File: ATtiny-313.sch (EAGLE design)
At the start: 16 parts, among them IC1 REG1117, IC2 ATtiny85

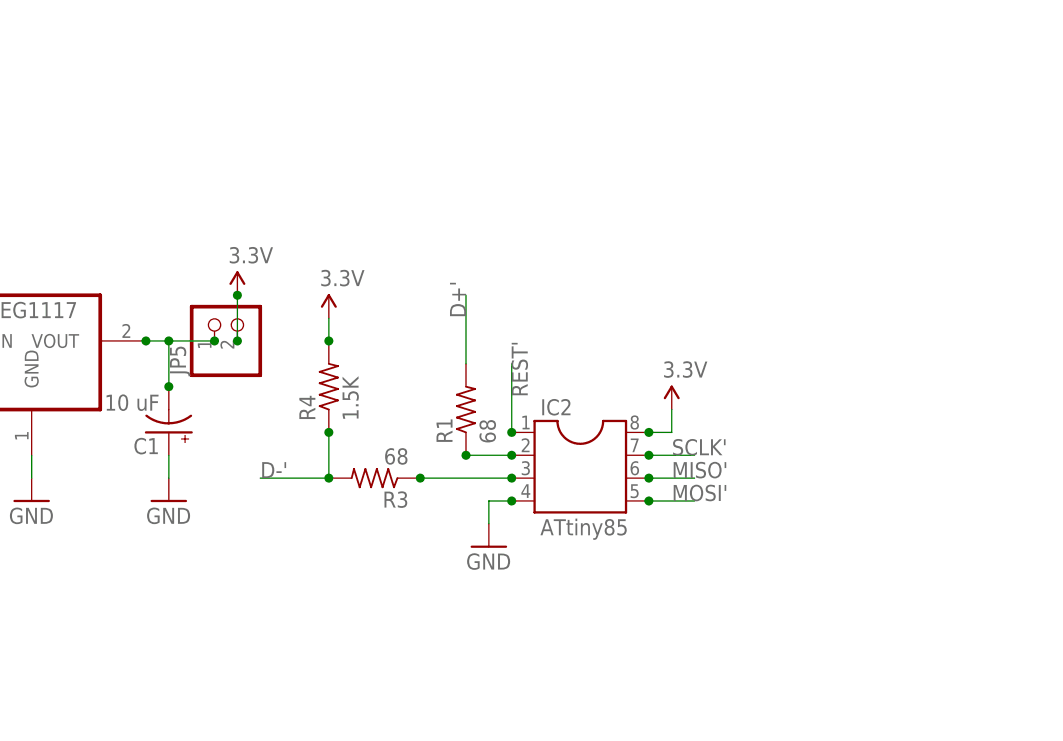
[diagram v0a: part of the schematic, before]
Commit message: more SMD goodness
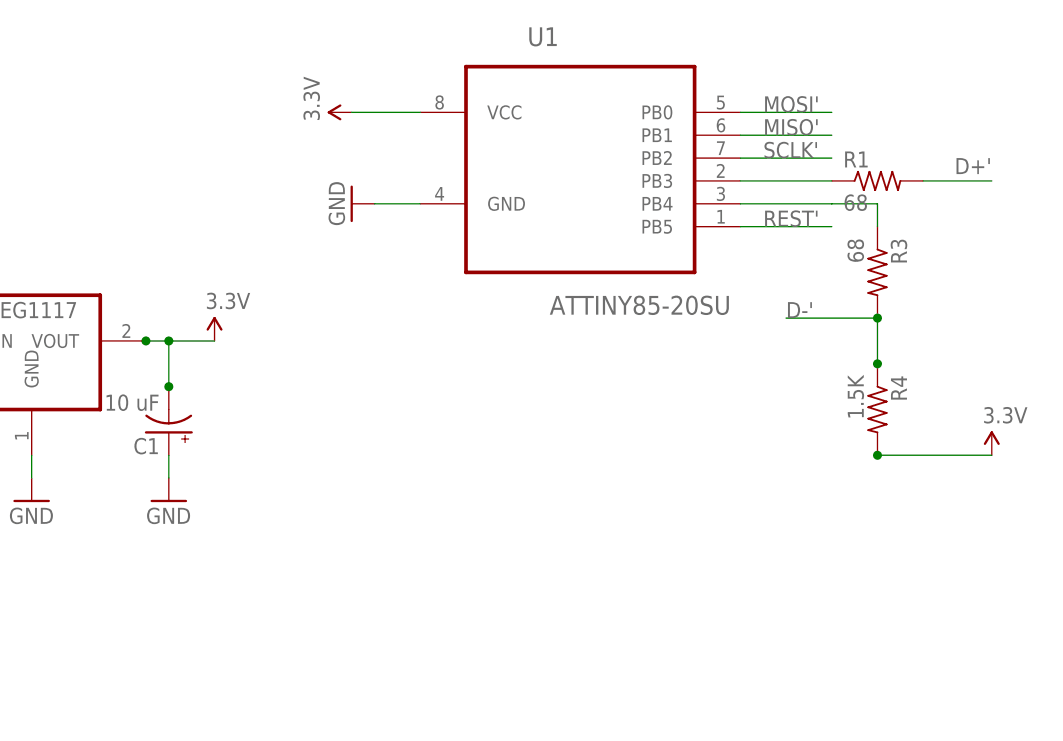
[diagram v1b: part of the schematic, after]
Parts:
- removed IC2: ATtiny85, ic-package:DIL8
- removed JP5: (no value), pinhead:PINHD-1X2
- added U1: ATTINY85-20SU, Atmel_By_element14_Batch_1:ATTINY85-20SU
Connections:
- removed net N$1: IC2.2, R1.1
- removed net N$2: IC2.3, R3.1
- removed net N$3: C1.-, IC1.VOUT, JP5.1
- new net N$15: R3.1, U1.PB4
- new net N$16: R1.1, U1.PB3
- net 3.3V: now also C1.-, IC1.VOUT, U1.VCC; no longer IC2.8, JP5.2
- net GND: now also U1.GND; no longer IC2.4
- net MISO': now also U1.PB1; no longer IC2.6
- net MOSI': now also U1.PB0; no longer IC2.5
- net REST': now also U1.PB5; no longer IC2.1
- net SCLK': now also U1.PB2; no longer IC2.7
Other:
- moved on the sheet: R1, R3, R4
